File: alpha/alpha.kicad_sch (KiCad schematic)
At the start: 34 parts, among them J1 Conn_01x02, J10 Conn_01x03, J2 Conn_01x02, J3 Conn_01x03, J4 Conn_01x03, J5 Conn_01x03, J6 Conn_01x03, J7 Conn_01x03, J8 Conn_01x03, J9 Conn_01x03, M1 Motor_AC_3_phase, M2 Motor_AC_3_phase, M3 Motor_AC_3_phase, M4 Motor_AC_3_phase, M5 CAM_servo, U1 Holybro Pixhawk 6X, U10 Radiomaster Bandit BR3 ELRS, U11 6V, 3A servo BEC, U12 5V, 5A step down converter, U13 Holybro Digital Air Speed Sen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, U14 Holybro I2C board, U15 Crazyflie Flow v2, U2 Holybro PM08D Power Module, U3 Holybro Tekko32 F4 Metal 4in1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, U4 iFlight Anti Spark Filter, U5 RFD868x, U6 Holybro M9N GPS, U7 3.3V, 0.6A step down converter, U8 Walksnail Avatar HD Pro Kit, U9 12V, 4.5A step down converter

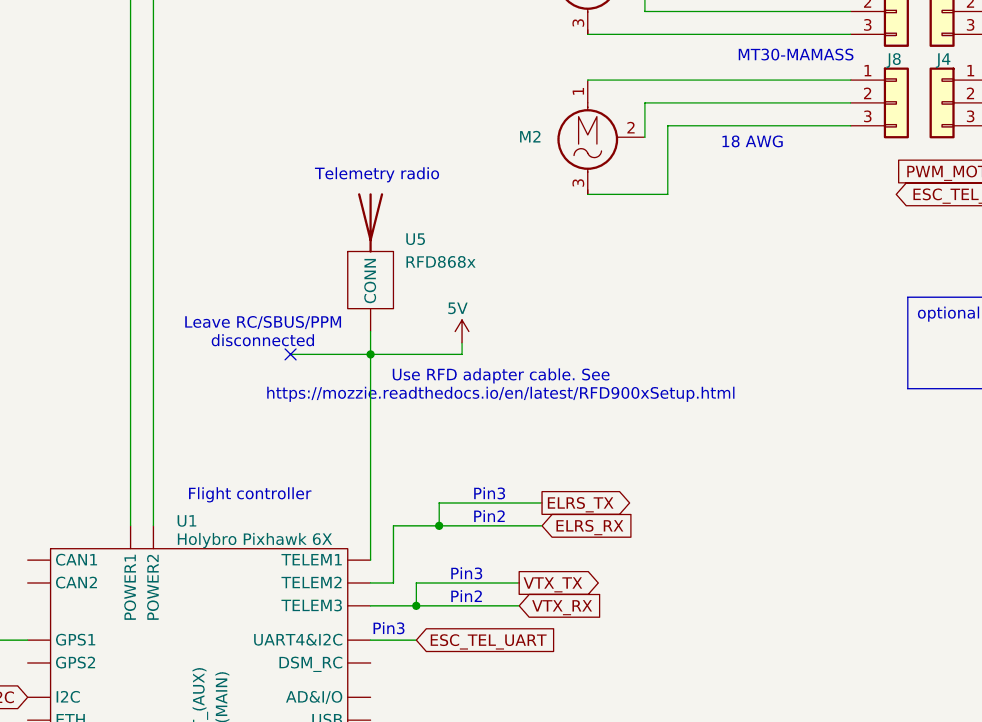
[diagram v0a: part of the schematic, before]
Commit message: update
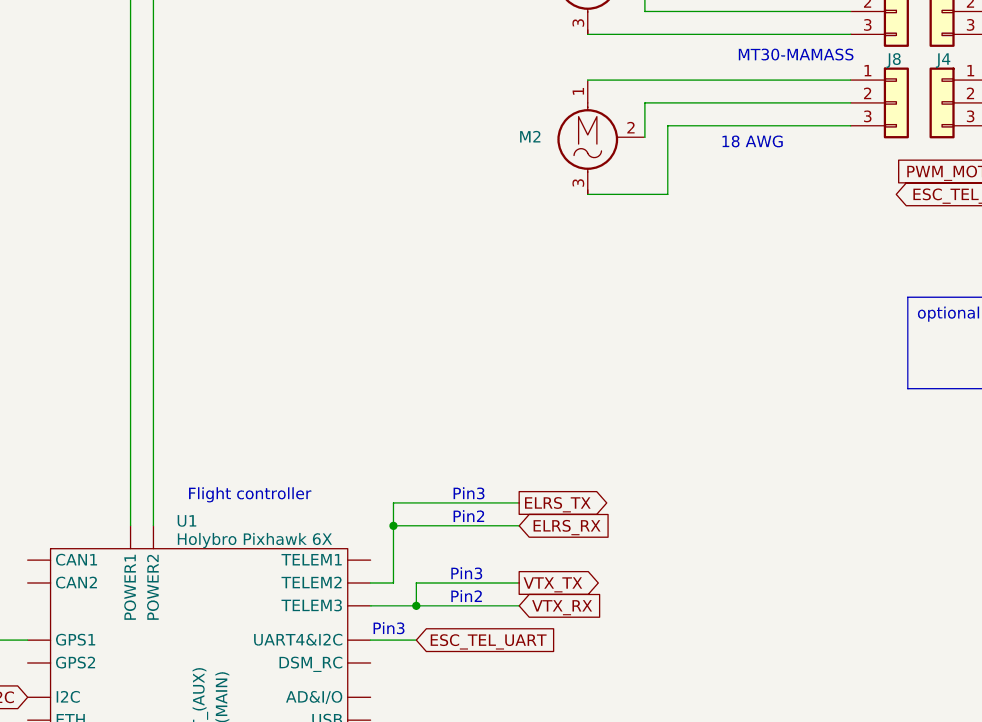
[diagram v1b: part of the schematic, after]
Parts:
- removed U5: RFD868x, symbol RF_Modules:RFD868x-EU_868Mhz_Long_Range
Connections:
- net 5V: no longer U1. (USB-C)
- net at U4. (OUT-): now also F1.2; no longer U2. (POWER2)
- new net: C1.1, C2.1, U11. (VOUT), U12. (VOUT), U2. (POWER2), U3. (VBAT), U7. (VOUT), U9. (VOUT)
- new net: U1. (USB-C), U2. (POWER2) (x2)
- new net: U2. (POWER2), U4. (OUT-) (x2)
- no-connect marks 4 -> 3
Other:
- note removed: "Leave RC/SBUS/PPM disconnected"
- note removed: "Telemetry radio"
- note removed: "Use RFD adapter cable. See https://mozzie.readthedocs.io/en/latest/RFD900xSetup.html"
